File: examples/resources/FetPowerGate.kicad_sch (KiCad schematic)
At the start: 7 parts

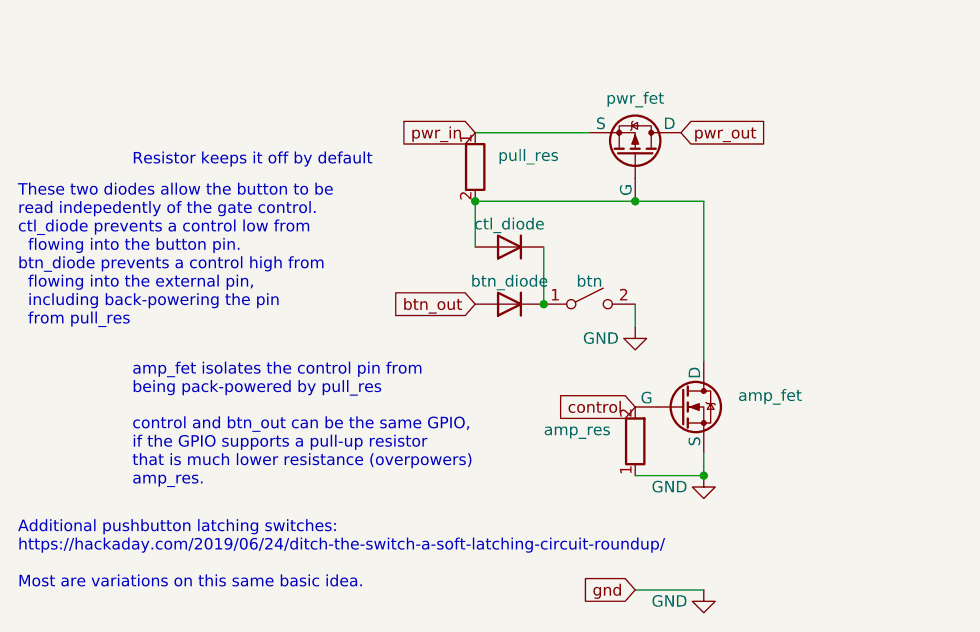
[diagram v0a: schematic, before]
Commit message: a version
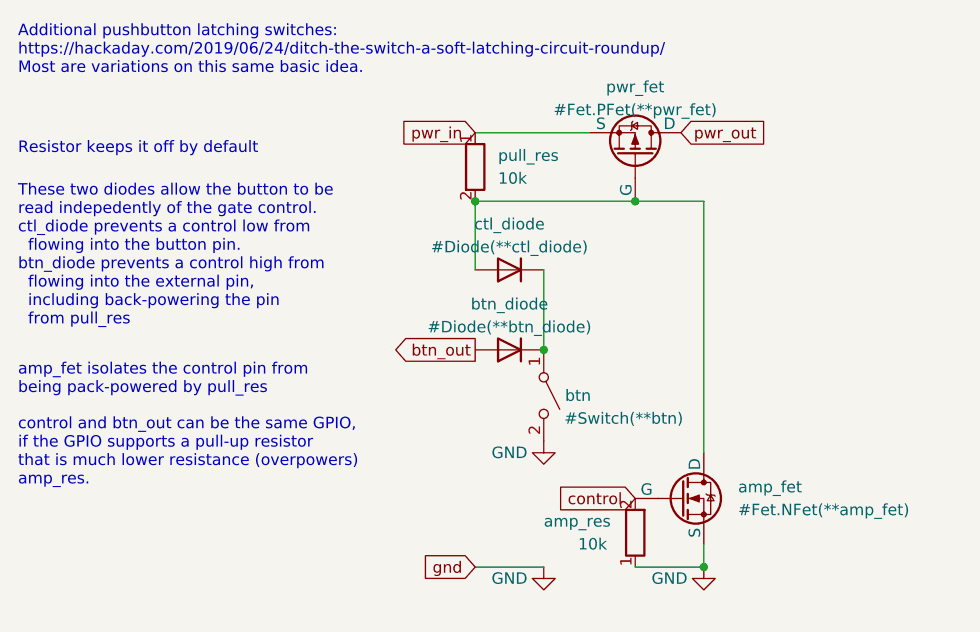
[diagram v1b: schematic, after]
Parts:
- amp_fet: value ~ -> #Fet.NFet(**amp_fet)
- amp_res, pull_res: value ~ -> 10k
- btn: value ~ -> #Switch(**btn)
- btn_diode: value ~ -> #Diode(**btn_diode)
- ctl_diode: value ~ -> #Diode(**ctl_diode)
- pwr_fet: value ~ -> #Fet.PFet(**pwr_fet)
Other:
- moved on the sheet: amp_fet, amp_res, btn, btn_diode, ctl_diode

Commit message: wip style
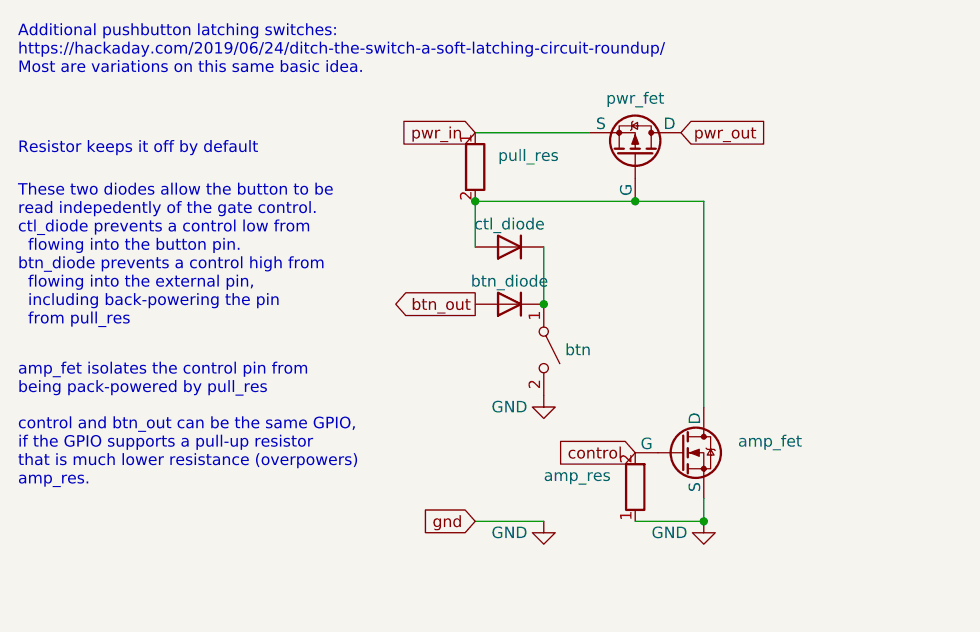
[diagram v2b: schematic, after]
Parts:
- amp_fet: value #Fet.NFet(**amp_fet) -> ~
- amp_res, pull_res: value 10k -> ~
- btn: value #Switch(**btn) -> ~
- btn_diode: value #Diode(**btn_diode) -> ~
- ctl_diode: value #Diode(**ctl_diode) -> ~
- pwr_fet: value #Fet.PFet(**pwr_fet) -> ~
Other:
- moved on the sheet: amp_fet, amp_res, btn, btn_diode, ctl_diode
